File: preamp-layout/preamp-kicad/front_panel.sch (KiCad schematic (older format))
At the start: 42 parts, among them J74 Conn_01x03_Female, J75 Conn_01x03_Female, J76 Conn_01x03_Female, J77 Conn_01x03_Female, J78 Conn_01x03_Female, J79 Conn_01x03_Female, J80 Conn_01x03_Female, J81 Conn_01x03_Female, J82 Conn_01x02_Male, J83 Conn_01x02_Male, J84 Conn_01x05_Female, SW11 Rotary_Encoder_Switch, SW12 Rotary_Encoder_Switch, U23 MCP23017_SO

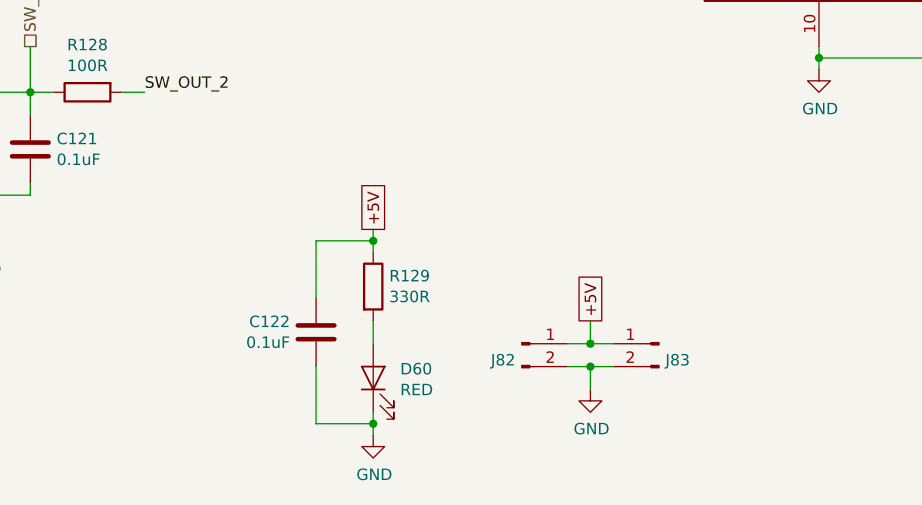
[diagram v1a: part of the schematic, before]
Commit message: PCB layout
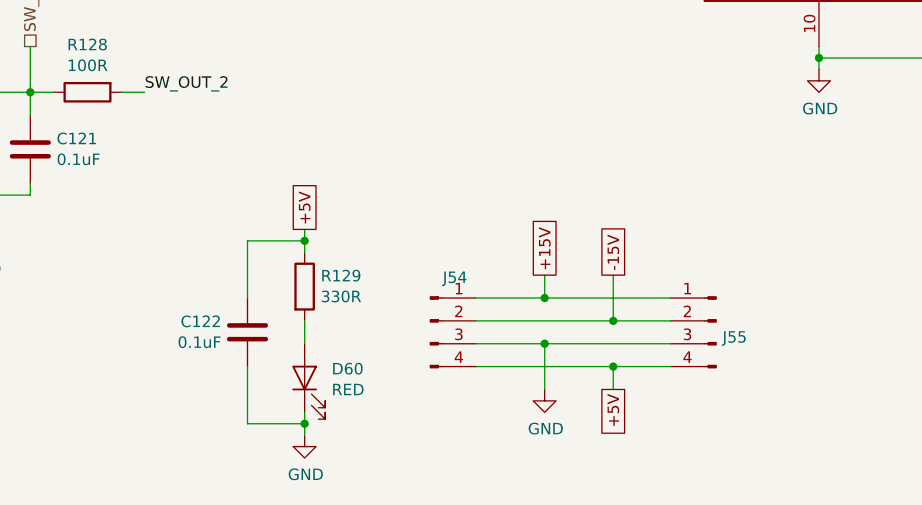
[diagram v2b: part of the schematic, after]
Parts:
- removed J82, J83: Conn_01x02_Male, Connector_JST:JST_EH_B2B-EH-A_1x02_P2.50mm_Vertical, symbol Connector:Conn_01x02_Male
- added J54, J55: Conn_01x04_Male, Connector_JST:JST_EH_S4B-EH_1x04_P2.50mm_Horizontal, symbol Connector:Conn_01x04_Male
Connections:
- net +5V: now also J54.4 (Pin_4), J55.4 (Pin_4)
- net GND: now also J54.3 (Pin_3), J55.3 (Pin_3)
- new net +15V: J54.1 (Pin_1), J55.1 (Pin_1)
- new net -15V: J54.2 (Pin_2), J55.2 (Pin_2)
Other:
- moved on the sheet: C122, D60, R129
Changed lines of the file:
@@
 L Device:R R?
 U 1 1 5ECB89C1
-P 4900 6700
+P 4600 6700
 AR Path="/5E2D8DA2/5ECB89C1" Ref="R?"  Part="1"
 AR Path="/5ECB89C1" Ref="R?"  Part="1"
@@
 AR Path="/5E5EF2D4/5ECB89C1" Ref="R?"  Part="1"
 AR Path="/5E5ECAAE/5ECB89C1" Ref="R129"  Part="1"
-F 0 "R129" H 4970 6746 50  0000 L CNN
-F 1 "330R" H 4970 6655 50  0000 L CNN
-F 2 "Resistor_SMD:R_1206_3216Metric_Pad1.42x1.75mm_HandSolder" V 4830 6700 50  0001 C CNN
-F 3 "~" H 4900 6700 50  0001 C CNN
-	1    4900 6700
-	1    0    0    -1
-$EndComp
-Text GLabel 4900 6450 1    50   UnSpc ~ 0
+F 0 "R129" H 4670 6746 50  0000 L CNN
+F 1 "330R" H 4670 6655 50  0000 L CNN
+F 2 "Resistor_SMD:R_1206_3216Metric_Pad1.42x1.75mm_HandSolder" V 4530 6700 50  0001 C CNN
+F 3 "~" H 4600 6700 50  0001 C CNN
+	1    4600 6700
+	1    0    0    -1
+$EndComp
+Text GLabel 4600 6450 1    50   UnSpc ~ 0
 +5V
 $Comp
 L power:GND #PWR?
 U 1 1 5ECB89D0
-P 4900 7350
+P 4600 7350
 AR Path="/5E26F6FE/5ECB89D0" Ref="#PWR?"  Part="1"
 AR Path="/5E5EF2D4/5ECB89D0" Ref="#PWR?"  Part="1"
 AR Path="/5E5ECAAE/5ECB89D0" Ref="#PWR0132"  Part="1"
-F 0 "#PWR0132" H 4900 7100 50  0001 C CNN
-F 1 "GND" H 4905 7177 50  0000 C CNN
-F 2 "" H 4900 7350 50  0001 C CNN
-F 3 "" H 4900 7350 50  0001 C CNN
-	1    4900 7350
-	1    0    0    -1
-$EndComp
-Wire Wire Line
-	4900 7250 4900 7300
-Wire Wire Line
-	4900 6850 4900 6950
-Wire Wire Line
-	4900 6450 4900 6500
+F 0 "#PWR0132" H 4600 7100 50  0001 C CNN
+F 1 "GND" H 4605 7177 50  0000 C CNN
+F 2 "" H 4600 7350 50  0001 C CNN
+F 3 "" H 4600 7350 50  0001 C CNN
+	1    4600 7350
+	1    0    0    -1
+$EndComp
+Wire Wire Line
+	4600 7250 4600 7300
+Wire Wire Line
+	4600 6850 4600 6950
+Wire Wire Line
+	4600 6450 4600 6500
 $Comp
 L Device:LED D?
 U 1 1 5ECB89C7
-P 4900 7100
+P 4600 7100
 AR Path="/5E2D8DA2/5ECB89C7" Ref="D?"  Part="1"
 AR Path="/5E27B612/5ECB89C7" Ref="D?"  Part="1"
 AR Path="/5E5EF2D4/5ECB89C7" Ref="D?"  Part="1"
 AR Path="/5E5ECAAE/5ECB89C7" Ref="D60"  Part="1"
-F 0 "D60" V 4939 6982 50  0000 R CNN
-F 1 "RED" V 4848 6982 50  0000 R CNN
-F 2 "LED_SMD:LED_1206_3216Metric_Pad1.42x1.75mm_HandSolder" H 4900 7100 50  0001 C CNN
-F 3 "~" H 4900 7100 50  0001 C CNN
-	1    4900 7100
+F 0 "D60" V 4639 6982 50  0000 R CNN
+F 1 "RED" V 4548 6982 50  0000 R CNN
+F 2 "LED_SMD:LED_1206_3216Metric_Pad1.42x1.75mm_HandSolder" H 4600 7100 50  0001 C CNN
+F 3 "~" H 4600 7100 50  0001 C CNN
+	1    4600 7100
 	0    -1   -1   0
 $EndComp
@@
 	9700 4650 9600 4650
 Wire Wire Line
-	4650 6750 4650 6500
-Connection ~ 4900 6500
-Wire Wire Line
-	4900 6500 4900 6550
-Wire Wire Line
-	4650 7050 4650 7300
-Connection ~ 4900 7300
-Wire Wire Line
-	4900 7300 4900 7350
+	4350 6750 4350 6500
+Connection ~ 4600 6500
+Wire Wire Line
+	4600 6500 4600 6550
+Wire Wire Line
+	4350 7050 4350 7300
+Connection ~ 4600 7300
+Wire Wire Line
+	4600 7300 4600 7350
 $Comp
 L Device:C C?
 U 1 1 5E8C1B16
-P 4650 6900
+P 4350 6900
 AR Path="/5E4A803E/5E8C1B16" Ref="C?"  Part="1"
 AR Path="/6009D432/5E8C1B16" Ref="C?"  Part="1"
 AR Path="/5E5ECAAE/5E8C1B16" Ref="C122"  Part="1"
-F 0 "C122" H 4536 6946 50  0000 R CNN
-F 1 "0.1uF" H 4536 6855 50  0000 R CNN
-F 2 "Capacitor_SMD:C_0805_2012Metric_Pad1.15x1.40mm_HandSolder" H 4688 6750 50  0001 C CNN
-F 3 "~" H 4650 6900 50  0001 C CNN
-	1    4650 6900
-	1    0    0    -1
-$EndComp
-Wire Wire Line
-	4650 6500 4900 6500
-Wire Wire Line
-	4650 7300 4900 7300
+F 0 "C122" H 4236 6946 50  0000 R CNN
+F 1 "0.1uF" H 4236 6855 50  0000 R CNN
+F 2 "Capacitor_SMD:C_0805_2012Metric_Pad1.15x1.40mm_HandSolder" H 4388 6750 50  0001 C CNN
+F 3 "~" H 4350 6900 50  0001 C CNN
+	1    4350 6900
+	1    0    0    -1
+$EndComp
+Wire Wire Line
+	4350 6500 4600 6500
+Wire Wire Line
+	4350 7300 4600 7300
 $Comp
 L Device:R R?
@@
 Wire Wire Line
 	7800 3250 7950 3250
-Wire Wire Line
-	5850 6950 5950 6950
-Connection ~ 5850 6950
-Wire Wire Line
-	5850 6850 5850 6950
-Connection ~ 5850 7050
-Wire Wire Line
-	5950 7050 5850 7050
-Wire Wire Line
-	5750 6950 5850 6950
-Wire Wire Line
-	5750 7050 5850 7050
-$Comp
-L Connector:Conn_01x02_Male J?
-U 1 1 60B80487
-P 6150 6950
-AR Path="/5E5EF2D4/60B80487" Ref="J?"  Part="1"
-AR Path="/6009D432/60B80487" Ref="J?"  Part="1"
-AR Path="/5E5ECAAE/60B80487" Ref="J83"  Part="1"
-F 0 "J83" H 6122 6878 50  0000 R CNN
-F 1 "Conn_01x02_Male" H 6122 6833 50  0001 R CNN
-F 2 "Connector_JST:JST_EH_B2B-EH-A_1x02_P2.50mm_Vertical" H 6150 6950 50  0001 C CNN
-F 3 "~" H 6150 6950 50  0001 C CNN
-	1    6150 6950
+$Comp
+L Connector:Conn_01x04_Male J?
+U 1 1 5FCE2A06
+P 5150 6850
+AR Path="/5E2D8DA2/5FCE2A06" Ref="J?"  Part="1"
+AR Path="/5E5ECAAE/5FCE2A06" Ref="J54"  Part="1"
+F 0 "J54" H 5258 7039 50  0000 C CNN
+F 1 "Conn_01x04_Male" H 5258 7040 50  0001 C CNN
+F 2 "Connector_JST:JST_EH_S4B-EH_1x04_P2.50mm_Horizontal" H 5150 6850 50  0001 C CNN
+F 3 "~" H 5150 6850 50  0001 C CNN
+	1    5150 6850
+	1    0    0    -1
+$EndComp
+$Comp
+L Connector:Conn_01x04_Male J?
+U 1 1 5FCE2A0C
+P 6400 6850
+AR Path="/5E2D8DA2/5FCE2A0C" Ref="J?"  Part="1"
+AR Path="/5E5ECAAE/5FCE2A0C" Ref="J55"  Part="1"
+F 0 "J55" H 6372 6778 50  0000 R CNN
+F 1 "Conn_01x04_Male" H 6508 7040 50  0001 C CNN
+F 2 "Connector_JST:JST_EH_S4B-EH_1x04_P2.50mm_Horizontal" H 6400 6850 50  0001 C CNN
+F 3 "~" H 6400 6850 50  0001 C CNN
+	1    6400 6850
 	-1   0    0    -1
 $EndComp
-Text GLabel 5850 6850 1    50   UnSpc ~ 0
+Wire Wire Line
+	5350 6750 5650 6750
+Wire Wire Line
+	5350 6850 5950 6850
+Text GLabel 5650 6650 1    50   UnSpc ~ 0
++15V
+Wire Wire Line
+	5650 6650 5650 6750
+Connection ~ 5650 6750
+Text GLabel 5950 6650 1    50   UnSpc ~ 0
+-15V
+Wire Wire Line
+	5950 7150 5950 7050
+Text GLabel 5950 7150 3    50   UnSpc ~ 0
 +5V
-Wire Wire Line
-	5850 7050 5850 7150
+Connection ~ 5950 7050
+Wire Wire Line
+	5950 7050 6200 7050
+Wire Wire Line
+	5650 6750 6200 6750
+Wire Wire Line
+	5350 7050 5950 7050
+Wire Wire Line
+	5350 6950 5650 6950
 $Comp
 L power:GND #PWR?
-U 1 1 64EC680F
-P 5850 7150
-AR Path="/5E26F6FE/64EC680F" Ref="#PWR?"  Part="1"
-AR Path="/5E5ECAAE/64EC680F" Ref="#PWR0133"  Part="1"
-F 0 "#PWR0133" H 5850 6900 50  0001 C CNN
-F 1 "GND" H 5855 6977 50  0000 C CNN
-F 2 "" H 5850 7150 50  0001 C CNN
-F 3 "" H 5850 7150 50  0001 C CNN
-	1    5850 7150
-	1    0    0    -1
-$EndComp
-$Comp
-L Connector:Conn_01x02_Male J?
-U 1 1 5E8B15E1
-P 5550 6950
-AR Path="/5E5EF2D4/5E8B15E1" Ref="J?"  Part="1"
-AR Path="/6009D432/5E8B15E1" Ref="J?"  Part="1"
-AR Path="/5E5ECAAE/5E8B15E1" Ref="J82"  Part="1"
-F 0 "J82" H 5522 6878 50  0000 R CNN
-F 1 "Conn_01x02_Male" H 5522 6833 50  0001 R CNN
-F 2 "Connector_JST:JST_EH_B2B-EH-A_1x02_P2.50mm_Vertical" H 5550 6950 50  0001 C CNN
-F 3 "~" H 5550 6950 50  0001 C CNN
-	1    5550 6950
-	1    0    0    -1
-$EndComp
+U 1 1 5FCE2A1F
+P 5650 7150
+AR Path="/6009D432/5FCE2A1F" Ref="#PWR?"  Part="1"
+AR Path="/5E2D8DA2/5FCE2A1F" Ref="#PWR?"  Part="1"
+AR Path="/5E5ECAAE/5FCE2A1F" Ref="#PWR048"  Part="1"
+F 0 "#PWR048" H 5650 6900 50  0001 C CNN
+F 1 "GND" H 5655 6977 50  0000 C CNN
+F 2 "" H 5650 7150 50  0001 C CNN
+F 3 "" H 5650 7150 50  0001 C CNN
+	1    5650 7150
+	1    0    0    -1
+$EndComp
+Wire Wire Line
+	5650 7150 5650 6950
+Connection ~ 5650 6950
+Wire Wire Line
+	5650 6950 6200 6950
+Wire Wire Line
+	5950 6650 5950 6850
+Connection ~ 5950 6850
+Wire Wire Line
+	5950 6850 6200 6850
 $EndSCHEMATC
